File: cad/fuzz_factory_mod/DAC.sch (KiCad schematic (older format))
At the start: 27 parts

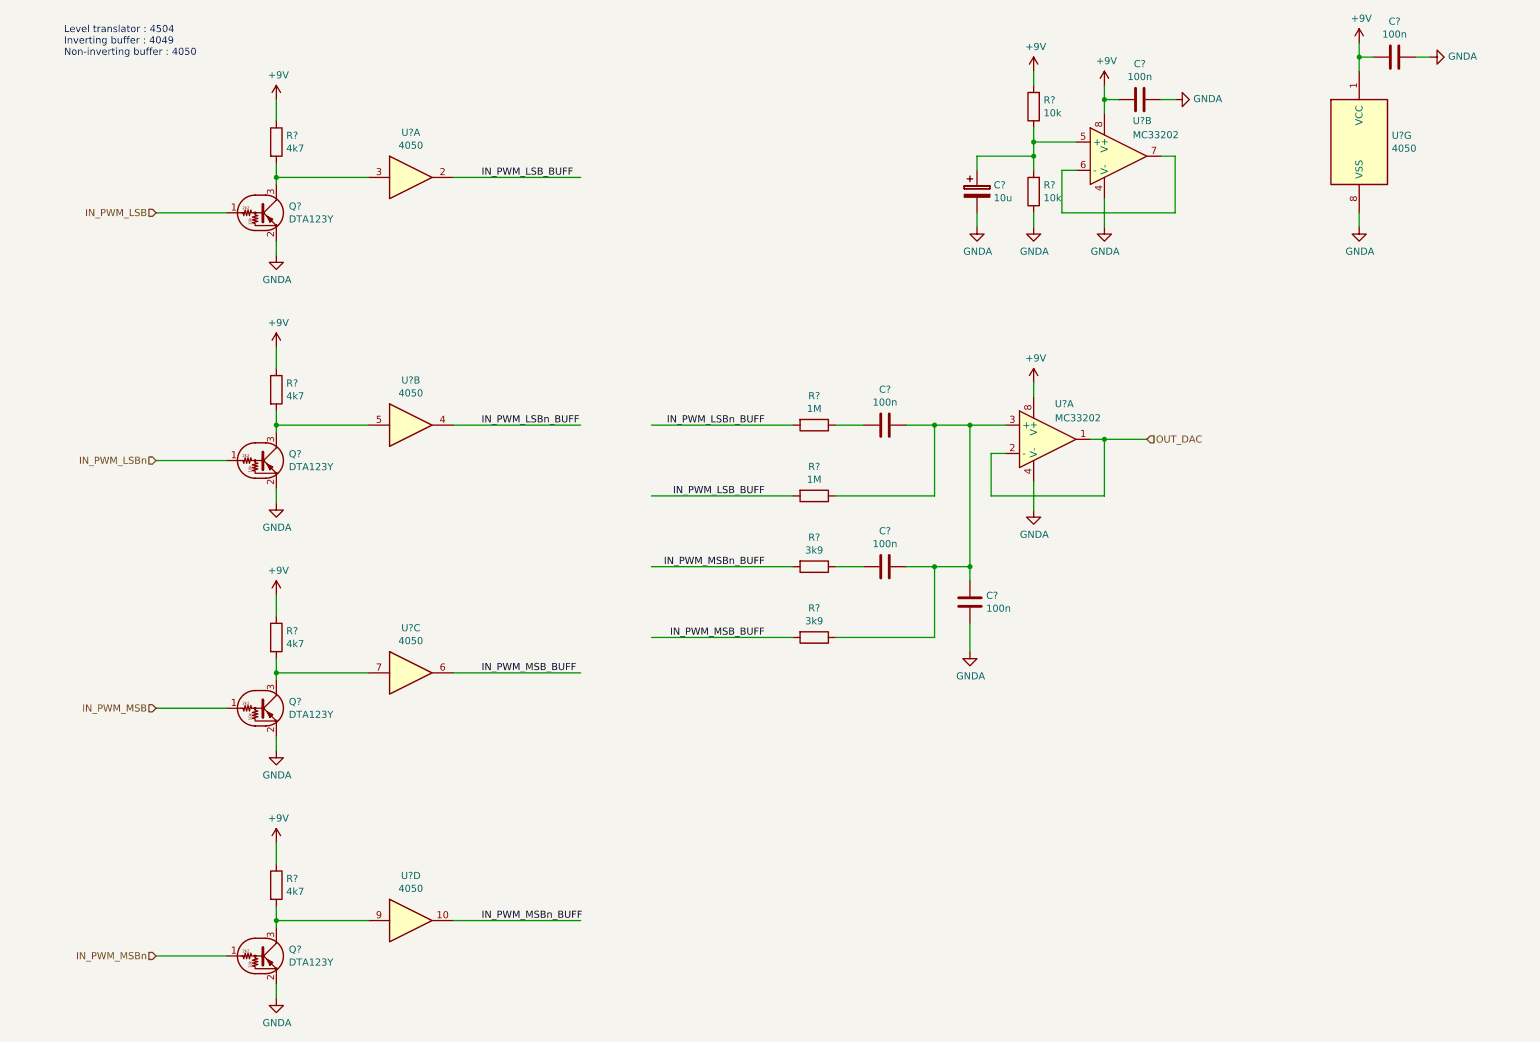
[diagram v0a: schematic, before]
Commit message: Continued schematic
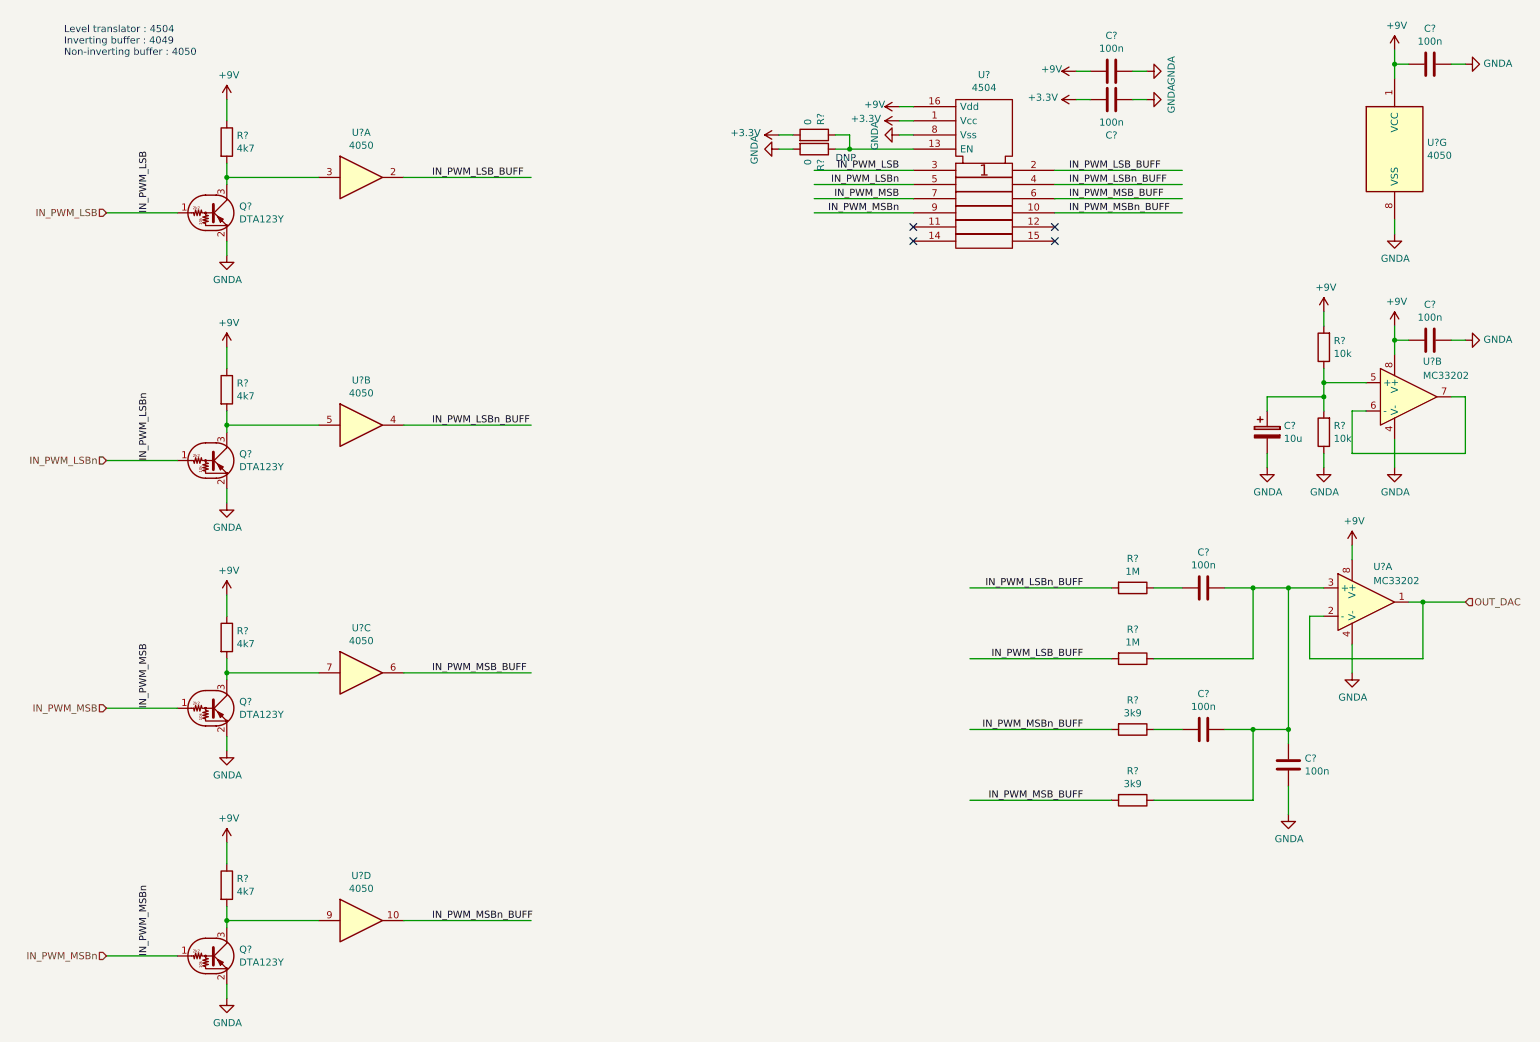
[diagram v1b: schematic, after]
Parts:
- added C? (x2): 100n, symbol Device:C
- added R? (x2): 0, symbol Device:R
- added U?: 4504, symbol 4xxx_IEEE:4504
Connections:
- net labels added: +3.3V
- wire segments 78 -> 99
- no-connect marks 0 -> 4
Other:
- note added: "DNP"
- moved on the sheet: C?, Q?, R?, U?A, U?B, U?C, U?D, U?G
